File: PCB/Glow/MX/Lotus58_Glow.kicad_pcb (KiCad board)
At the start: 2 copper layers, 139.1 x 106.7 mm, 122 parts, among them J1 AudioJack4, P4 OLED, SW1 SW_PUSH, SW10 SW_PUSH, SW11 SW_PUSH, SW12 SW_PUSH, SW13 SW_PUSH, SW14 SW_PUSH, SW15 SW_PUSH, SW16 SW_PUSH, SW17 SW_PUSH, SW18 SW_PUSH, SW19 SW_PUSH, SW2 SW_PUSH, SW20 SW_PUSH, SW21 SW_PUSH, SW22 SW_PUSH, SW23 SW_PUSH, SW24 SW_PUSH, SW25 SW_PUSH, SW26 SW_PUSH, SW27 SW_PUSH, SW28 SW_PUSH, SW29 SW_PUSH, SW3 SW_PUSH, SW30 Rotary_Encoder_Switch, SW31 Rotary_Encoder_Switch, SW4 SW_PUSH, SW5 SW_PUSH, SW6 SW_PUSH, SW7 SW_PUSH, SW8 SW_PUSH, SW9 SW_PUSH, U1 ProMicro

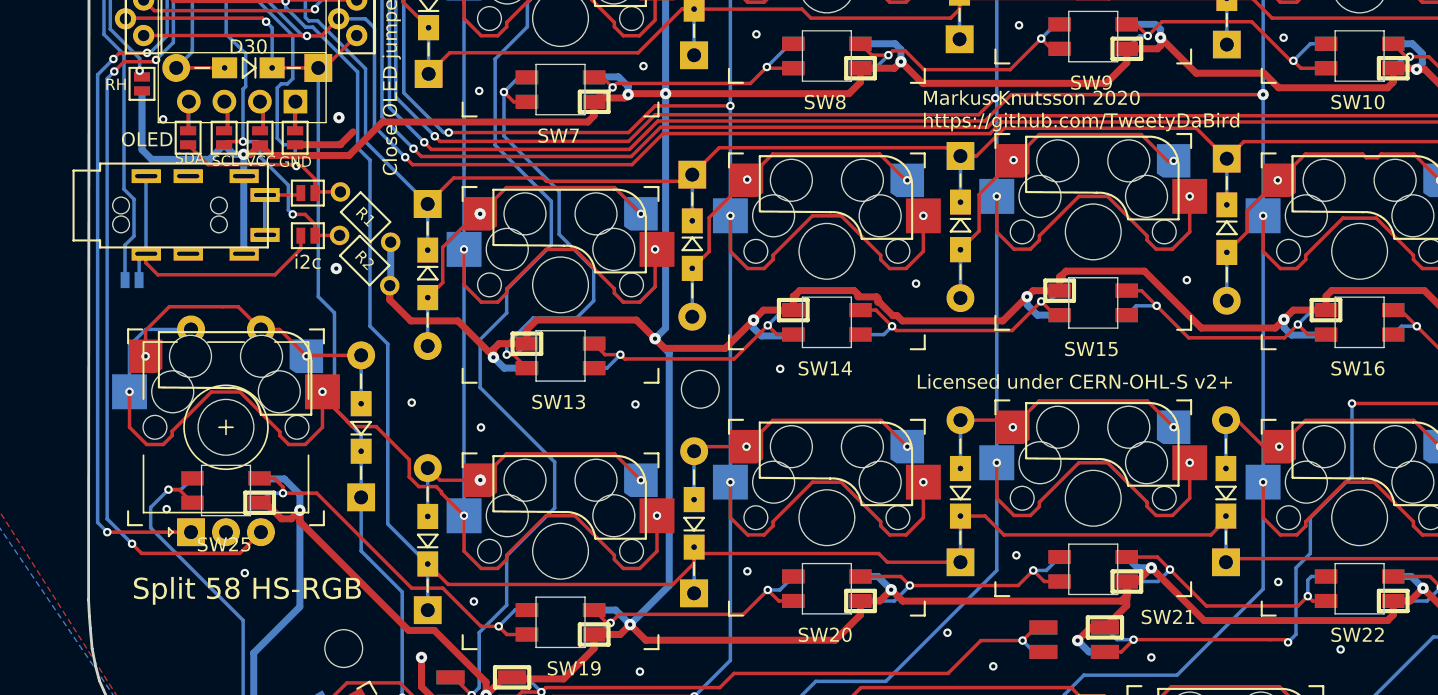
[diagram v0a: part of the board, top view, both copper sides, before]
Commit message: Updated silkscreen
New name!
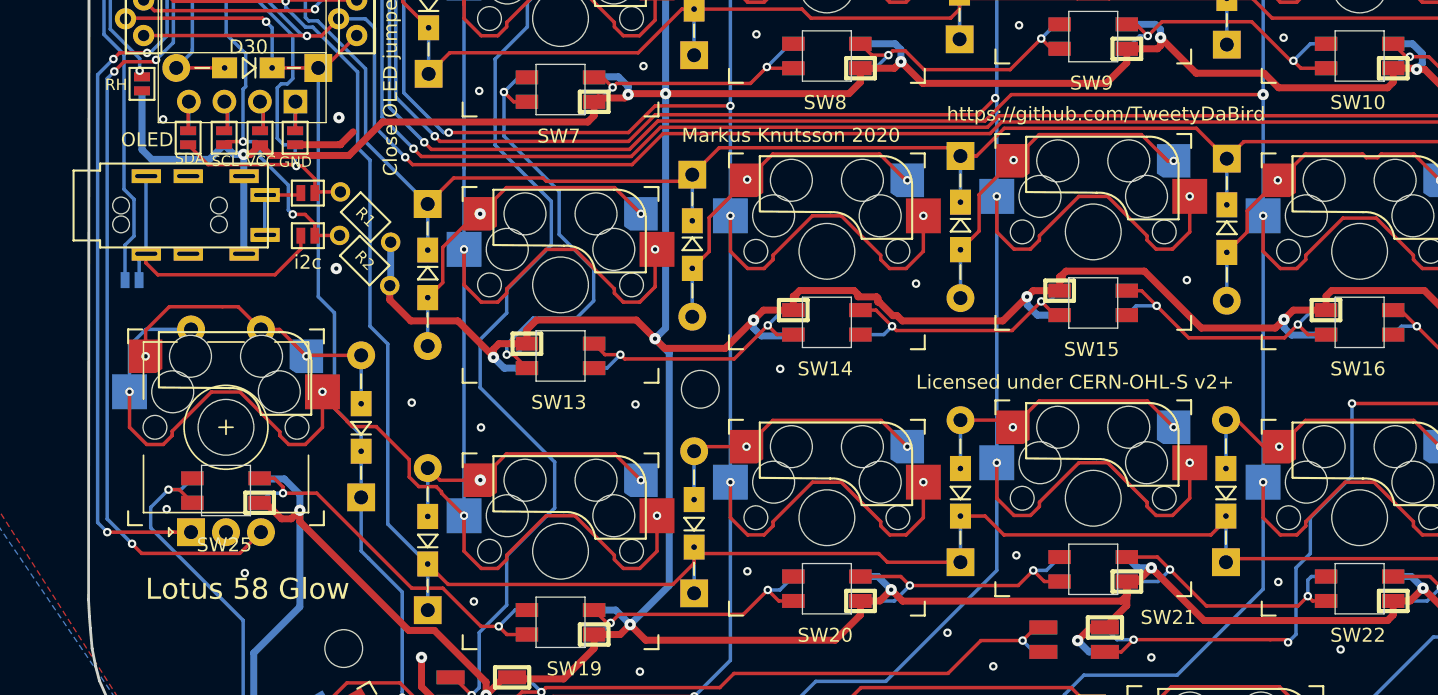
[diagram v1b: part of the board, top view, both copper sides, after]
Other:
- board text added: "Lotus 58 Glow"
- board text added: "Markus Knutsson 2020"
- board text added: "https://github.com/TweetyDaBird"
- board text removed: "Markus Knutsson 2020 https://github.com/TweetyDaBird"
- board text removed: "Split 58 HS-RGB"
